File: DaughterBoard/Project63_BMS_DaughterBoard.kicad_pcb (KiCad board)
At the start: 4 copper layers, 147.8 x 100.5 mm, 166 parts, among them J1 430450200, J4 1-794106-0, J5 430450200, Q1 ZXTN4004KTC, U1 BQ79614PAPRQ1

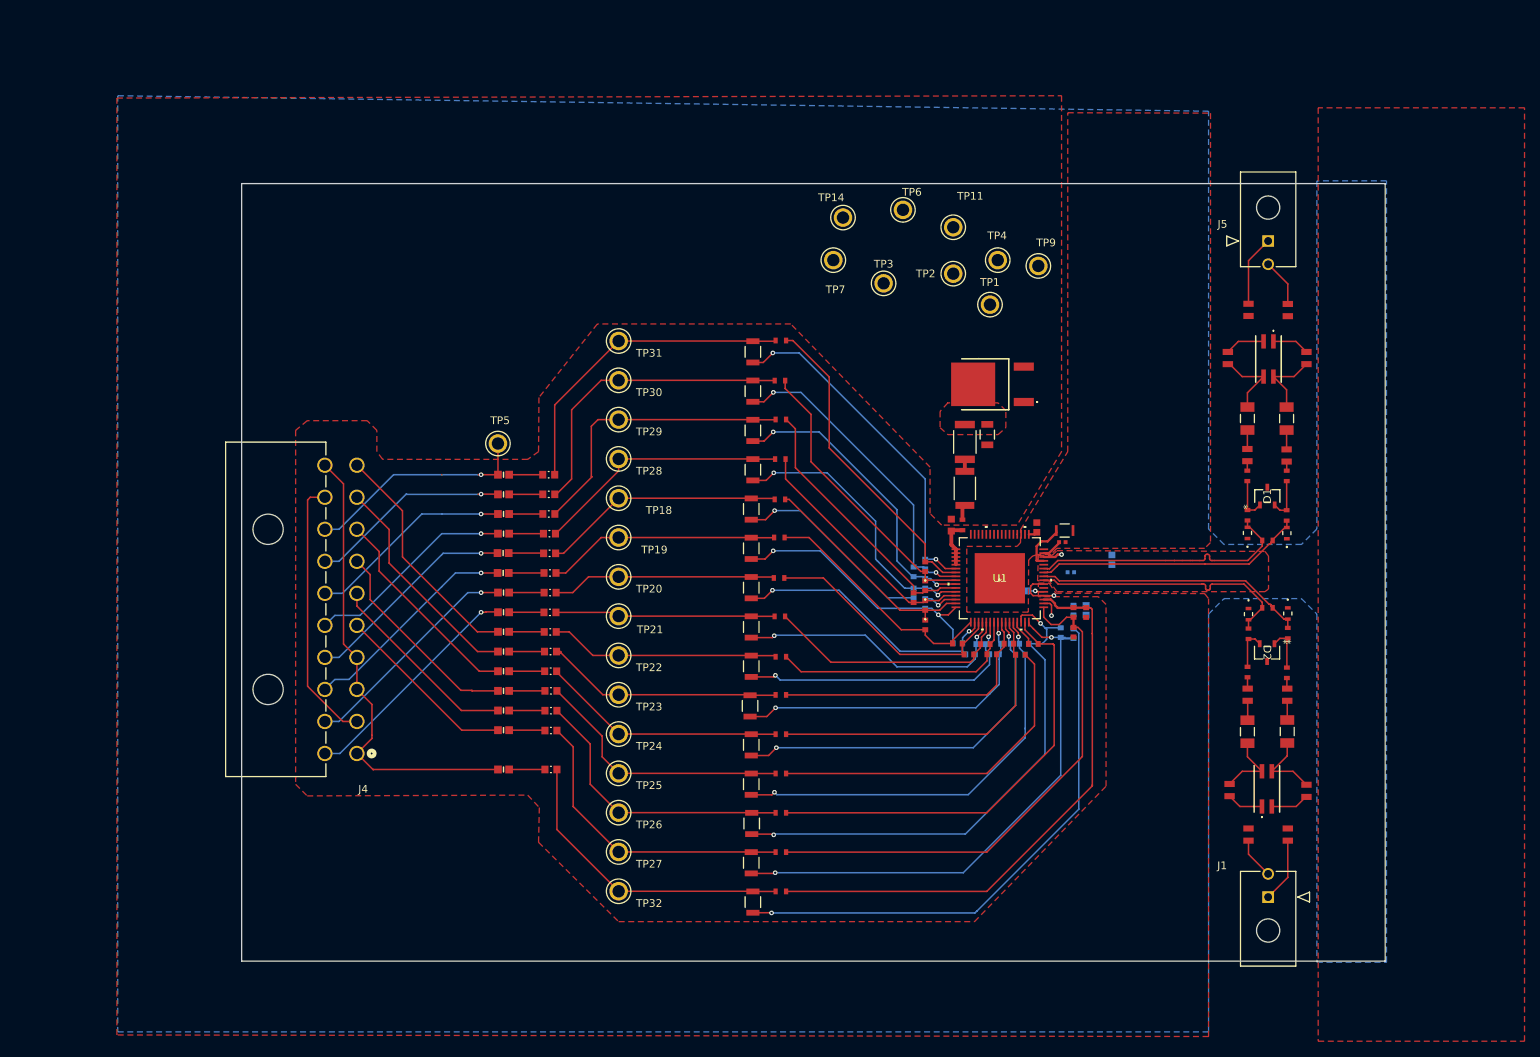
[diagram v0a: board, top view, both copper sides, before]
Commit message: Finished board
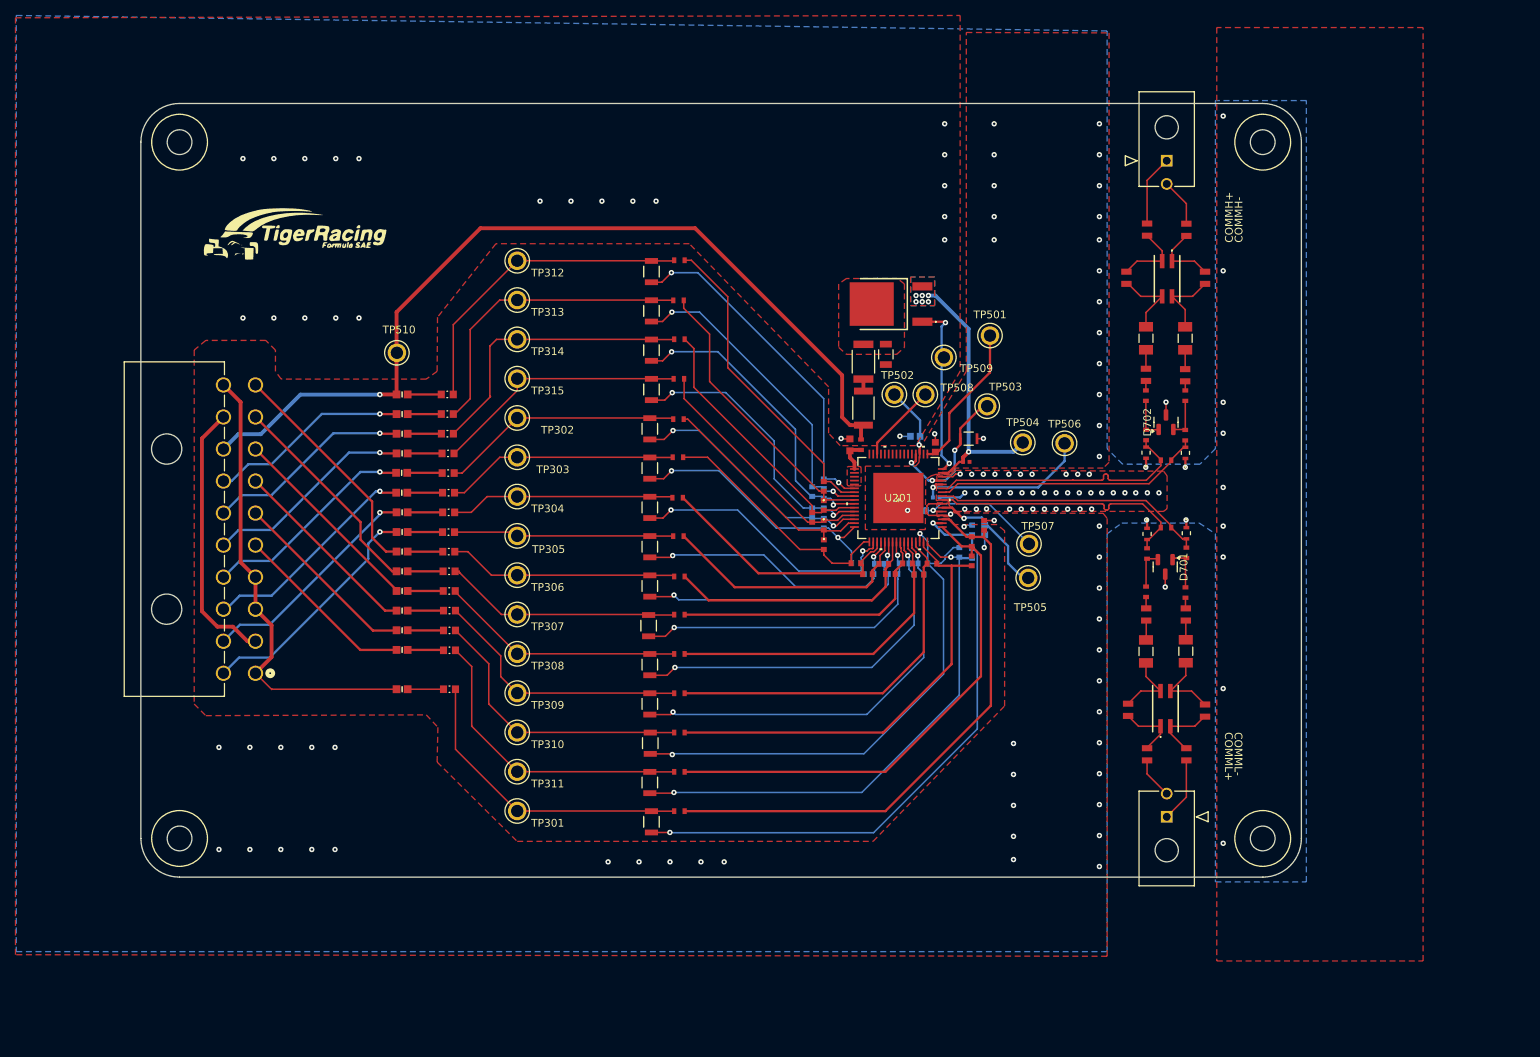
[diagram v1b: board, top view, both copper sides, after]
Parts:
- removed D1, D2: 24V, PESD1CAN_215:SOT23_PESD1_NEX
- added D701: 24V, Package_TO_SOT_SMD:SOT-23, F.Cu at (197.4, 94.9)
- added D702: 24V, Package_TO_SOT_SMD:SOT-23, F.Cu at (197.5, 76.2)
- added G***: LOGO, LOGO, F.Cu at (84.9, 51.9)
- added H101: MountingHole, MountingHole:MountingHole_3.2mm_M3, F.Cu at (70.0, 40.0)
- added H102: MountingHole, MountingHole:MountingHole_3.2mm_M3, F.Cu at (210.0, 40.0)
- added H103: MountingHole, MountingHole:MountingHole_3.2mm_M3, F.Cu at (70.0, 130.0)
- added H104: MountingHole, MountingHole:MountingHole_3.2mm_M3, F.Cu at (210.0, 130.0)
- moved TP505 48.2 mm to (179.7, 96.3)
- moved TP507 46.1 mm to (179.8, 91.9)
- moved TP506 31.2 mm to (184.4, 78.9)
- moved C205 30.0 mm to (165.1, 78.0), turned to 0 degrees
- moved TP508 25.2 mm to (166.4, 72.6)
- moved TP504 23.6 mm to (179.0, 78.8)
- moved C202 19.9 mm to (167.8, 85.9)
- moved TP503 19.3 mm to (174.4, 74.1)
- moved TP510 17.6 mm to (98.1, 67.2)
- moved C322 17.3 mm to (174.0, 89.5), turned to -90 degrees
- moved C206 17.2 mm to (172.0, 78.3)
- moved TP502 17.0 mm to (162.4, 72.6)
- moved C303 16.7 mm to (159.1, 95.8)
- moved C308 16.7 mm to (166.1, 94.5)
- moved C313 16.7 mm to (157.4, 94.4)
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- renumbered C1 to C201, C2 to C202, C3 to C203, C4 to C204, C5 to C205, C6 to C206, C7 to C207, C8 to C208, C9 to C301, C10 to C302, C11 to C303, C12 to C304, C13 to C305, C14 to C306, C15 to C307, C16 to C308, C17 to C309, C18 to C310, C19 to C311, C20 to C312, C21 to C313, C22 to C314, C23 to C315, C24 to C316, C25 to C317, C26 to C318, C27 to C319, C28 to C320, C29 to C321, C30 to C322, C31 to C323, C32 to C324, C33 to C325, C34 to C326, C35 to C327, C36 to C328, C37 to C329, C38 to C330, C39 to C601, C44 to C701, C43 to C702, C41 to C703, C40 to C704, C45 to C705, C42 to C706, C46 to C707, C47 to C708, F26 to F301, F25 to F302, F24 to F303, F23 to F304, F22 to F305, F21 to F306, F20 to F307, F19 to F308, F18 to F309, F17 to F310, F16 to F311, F11 to F312, F10 to F313, F9 to F314, F8 to F315, F7 to F316, F2 to F317, F6 to F318, F5 to F319, F4 to F320, F3 to F321, F1 to F322, F30 to F323, F29 to F324, F28 to F325, F27 to F326, F15 to F327, F14 to F328, F13 to F329, F12 to F330, FL1 to FL701, FL2 to FL702, J4 to J401, J1 to J701, J5 to J702, Q1 to Q601, R1 to R201, R2 to R301, R3 to R302, R4 to R303, R5 to R304, R6 to R305, R7 to R306, R8 to R307, R9 to R308, R10 to R309, R11 to R310, R12 to R311, R13 to R312, R14 to R313, R15 to R314, R16 to R315, R17 to R316, R18 to R317, R19 to R318, R20 to R319, R21 to R320, R22 to R321, R23 to R322, R27 to R323, R26 to R324, R25 to R325, R24 to R326, R29 to R327, R30 to R328, R31 to R329, R28 to R330, R32 to R601, R33 to R602, R43 to R701, R44 to R702, R37 to R703, R38 to R704, R47 to R705, R48 to R706, R34 to R707, R35 to R708, R45 to R709, R46 to R710, R36 to R711, R49 to R712, R54 to R713, R55 to R714, R52 to R715, R53 to R716, R41 to R717, R42 to R718, R40 to R719, R39 to R720, R50 to R721, R51 to R722, TP32 to TP301, TP18 to TP302, TP19 to TP303, TP20 to TP304, TP21 to TP305, TP22 to TP306, TP23 to TP307, TP24 to TP308, TP25 to TP309, TP26 to TP310, TP27 to TP311, TP31 to TP312, TP30 to TP313, TP29 to TP314, TP28 to TP315, TP11 to TP501, TP1 to TP502, TP9 to TP503, TP2 to TP504, TP7 to TP505, TP3 to TP506, TP6 to TP507, TP14 to TP508, TP4 to TP509, TP5 to TP510, U1 to U201
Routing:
- net BAT: track 31.7 -> 116.5 mm
- net LDOIN: track 2.64 -> 35.2 mm, vias 0 -> 7
- net NEG5V: track 0.00 -> 23.3 mm, vias 0 -> 1
- net NPNB: track 0.00 -> 23.0 mm, vias 0 -> 2
- net AVSS: track 9.41 -> 29.8 mm, vias 2 -> 132
- net DVDD: track 1.14 -> 18.9 mm
- net AVDD: track 0.31 -> 15.9 mm, vias 0 -> 1
- net REFHP: track 2.22 -> 17.1 mm
- net CVDD: track 6.38 -> 20.6 mm, vias 0 -> 3
- net NFAULT: track 0.00 -> 10.3 mm
- net TSREF: track 0.00 -> 8.97 mm, vias 0 -> 1
- net CB0: track 74.2 -> 79.9 mm
- net Net-(FL702-N2+): track 5.22 -> 9.27 mm
- net Net-(FL702-N1+): track 4.84 -> 8.87 mm
- net Net-(FL701-N2+): track 4.99 -> 8.55 mm
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- added copper zone on F.Cu, net /BQ79614_Bootstrapping/Cell 14S PIN
- added copper zone on In2.Cu, net AVSS
- added copper zone on B.Cu, net LDOIN
- added copper zone on F.Cu, net LDOIN
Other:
- board size 147.8 x 100.5 mm -> 150 x 100 mm
- board text added: "COMMH+"
- board text added: "COMMH-"
- board text added: "COMML+"
- board text added: "COMML-"
